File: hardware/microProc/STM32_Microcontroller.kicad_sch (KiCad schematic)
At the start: 11 parts, among them U1 STM32L021K4Tx

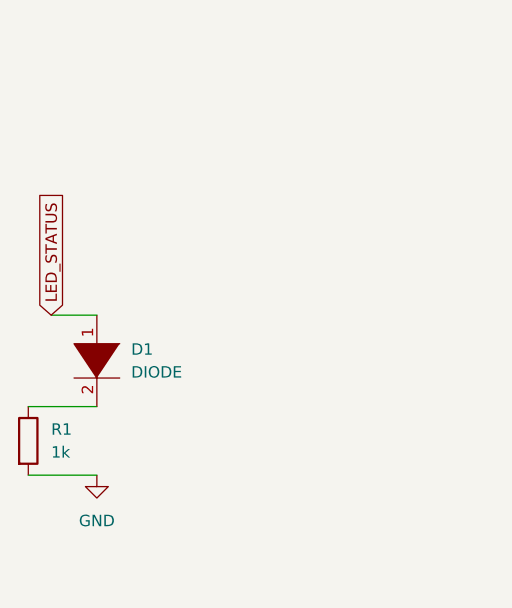
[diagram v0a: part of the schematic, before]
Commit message: Component placement
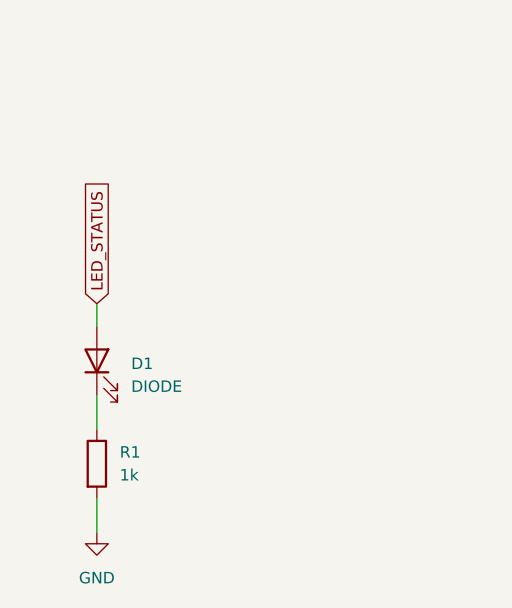
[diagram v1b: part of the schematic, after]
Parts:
- D1: symbol pspice:DIODE -> Device:LED
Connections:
- net LED_STATUS: now also D1.2 (A); no longer D1.1 (K)
- net at R1.1: now also D1.1 (K); no longer D1.2 (A)
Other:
- moved on the sheet: D1, R1
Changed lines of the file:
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@@
     (stroke (width 0) (type default) (color 0 0 0 0))
   )
-  (wire (pts (xy 59.69 109.22) (xy 64.77 109.22))
+  (wire (pts (xy 64.77 107.95) (xy 64.77 110.49))
     (stroke (width 0) (type default) (color 0 0 0 0))
   )
@@
     (stroke (width 0) (type default) (color 0 0 0 0))
   )
-  (wire (pts (xy 57.15 119.38) (xy 64.77 119.38))
-    (stroke (width 0) (type default) (color 0 0 0 0))
-  )
-  (wire (pts (xy 57.15 127) (xy 64.77 127))
+  (wire (pts (xy 64.77 118.11) (xy 64.77 121.92))
+    (stroke (width 0) (type default) (color 0 0 0 0))
+  )
+  (wire (pts (xy 64.77 129.54) (xy 64.77 133.35))
     (stroke (width 0) (type default) (color 0 0 0 0))
   )
@@
     )
   )
-  (global_label "LED_STATUS" (shape input) (at 59.69 109.22 90) (fields_autoplaced)
-    (effects (font (size 1.27 1.27)) (justify left))
-    (property "Intersheet References" "${INTERSHEET_REFS}" (id 0) (at 59.6106 95.6188 90)
+  (global_label "LED_STATUS" (shape input) (at 64.77 107.95 90) (fields_autoplaced)
+    (effects (font (size 1.27 1.27)) (justify left))
+    (property "Intersheet References" "${INTERSHEET_REFS}" (id 0) (at 64.6906 94.3488 90)
       (effects (font (size 1.27 1.27)) (justify left) hide)
     )
@@
     (pin "1")
   )
-  (symbol (lib_id "Device:R") (at 57.15 123.19 0) (unit 1)
-    (in_bom yes) (on_board yes) (fields_autoplaced)
-    (property "Reference" "R1" (id 0) (at 59.69 121.9199 0)
-      (effects (font (size 1.27 1.27)) (justify left))
-    )
-    (property "Value" "1k" (id 1) (at 59.69 124.4599 0)
-      (effects (font (size 1.27 1.27)) (justify left))
-    )
-    (property "Footprint" "Resistor_SMD:R_0805_2012Metric_Pad1.20x1.40mm_HandSolder" (id 2) (at 55.372 123.19 90)
-      (effects (font (size 1.27 1.27)) hide)
-    )
-    (property "Datasheet" "~" (id 3) (at 57.15 123.19 0)
+  (symbol (lib_id "Device:R") (at 64.77 125.73 0) (unit 1)
+    (in_bom yes) (on_board yes) (fields_autoplaced)
+    (property "Reference" "R1" (id 0) (at 67.31 124.4599 0)
+      (effects (font (size 1.27 1.27)) (justify left))
+    )
+    (property "Value" "1k" (id 1) (at 67.31 126.9999 0)
+      (effects (font (size 1.27 1.27)) (justify left))
+    )
+    (property "Footprint" "Resistor_SMD:R_0805_2012Metric_Pad1.20x1.40mm_HandSolder" (id 2) (at 62.992 125.73 90)
+      (effects (font (size 1.27 1.27)) hide)
+    )
+    (property "Datasheet" "~" (id 3) (at 64.77 125.73 0)
       (effects (font (size 1.27 1.27)) hide)
     )
@@
     (pin "2")
   )
-  (symbol (lib_id "power:GND") (at 64.77 127 0) (unit 1)
-    (in_bom yes) (on_board yes) (fields_autoplaced)
-    (property "Reference" "#PWR01" (id 0) (at 64.77 133.35 0)
-      (effects (font (size 1.27 1.27)) hide)
-    )
-    (property "Value" "GND" (id 1) (at 64.77 132.08 0))
-    (property "Footprint" "" (id 2) (at 64.77 127 0)
-      (effects (font (size 1.27 1.27)) hide)
-    )
-    (property "Datasheet" "" (id 3) (at 64.77 127 0)
+  (symbol (lib_id "power:GND") (at 64.77 133.35 0) (unit 1)
+    (in_bom yes) (on_board yes) (fields_autoplaced)
+    (property "Reference" "#PWR01" (id 0) (at 64.77 139.7 0)
+      (effects (font (size 1.27 1.27)) hide)
+    )
+    (property "Value" "GND" (id 1) (at 64.77 138.43 0))
+    (property "Footprint" "" (id 2) (at 64.77 133.35 0)
+      (effects (font (size 1.27 1.27)) hide)
+    )
+    (property "Datasheet" "" (id 3) (at 64.77 133.35 0)
       (effects (font (size 1.27 1.27)) hide)
     )
@@
     (pin "1")
   )
-  (symbol (lib_id "pspice:DIODE") (at 64.77 114.3 270) (unit 1)
-    (in_bom yes) (on_board yes) (fields_autoplaced)
-    (property "Reference" "D1" (id 0) (at 68.58 113.0299 90)
-      (effects (font (size 1.27 1.27)) (justify left))
-    )
-    (property "Value" "DIODE" (id 1) (at 68.58 115.5699 90)
-      (effects (font (size 1.27 1.27)) (justify left))
+  (symbol (lib_id "Device:LED") (at 64.77 114.3 90) (unit 1)
+    (in_bom yes) (on_board yes) (fields_autoplaced)
+    (property "Reference" "D1" (id 0) (at 68.58 114.6174 90)
+      (effects (font (size 1.27 1.27)) (justify right))
+    )
+    (property "Value" "DIODE" (id 1) (at 68.58 117.1574 90)
+      (effects (font (size 1.27 1.27)) (justify right))
     )
     (property "Footprint" "LED_SMD:LED_0603_1608Metric_Pad1.05x0.95mm_HandSolder" (id 2) (at 64.77 114.3 0)
